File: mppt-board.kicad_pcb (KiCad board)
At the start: 6 copper layers, 46.5 x 49 mm, 29 parts, among them J1 Out, J2 programming, Q1 IPD25N06S4L30ATMA2, U1 MC33201DR2G, U2 LM3671, U3 STM32G030J6Mx

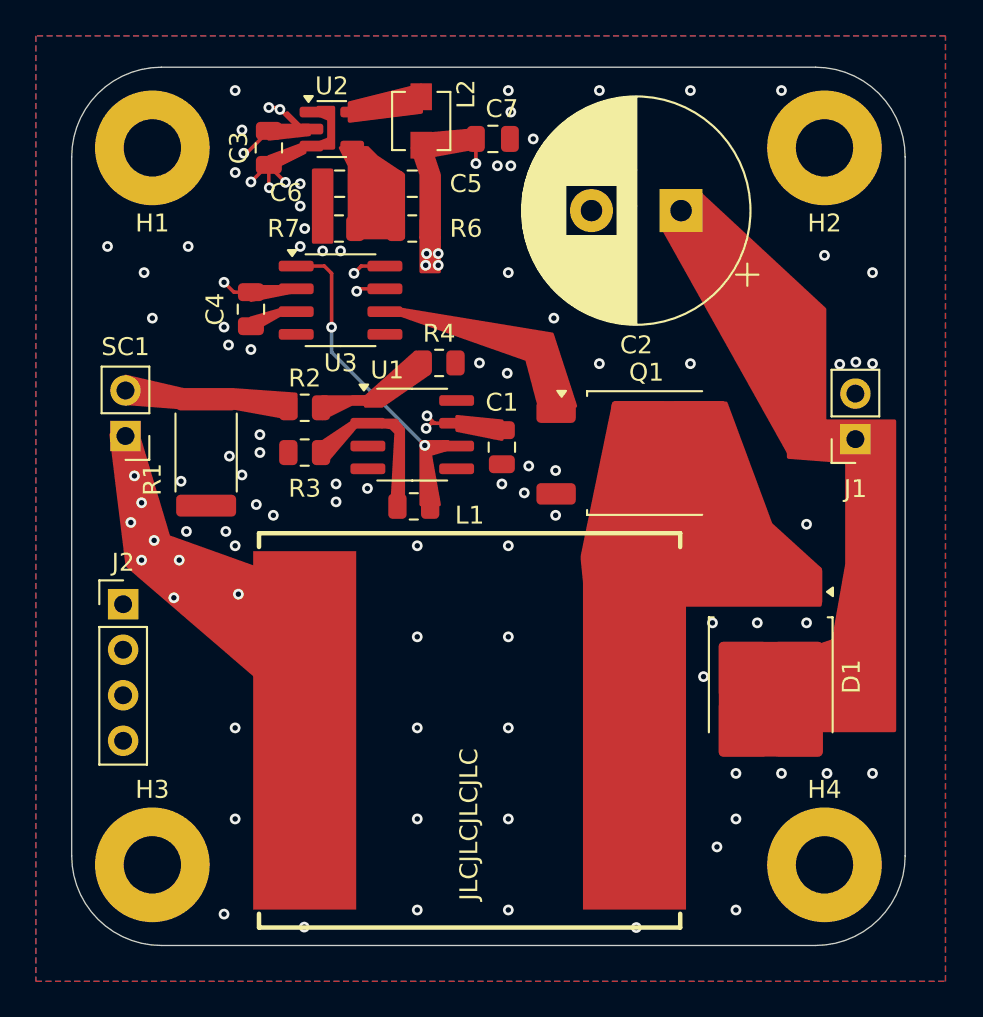
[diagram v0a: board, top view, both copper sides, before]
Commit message: init
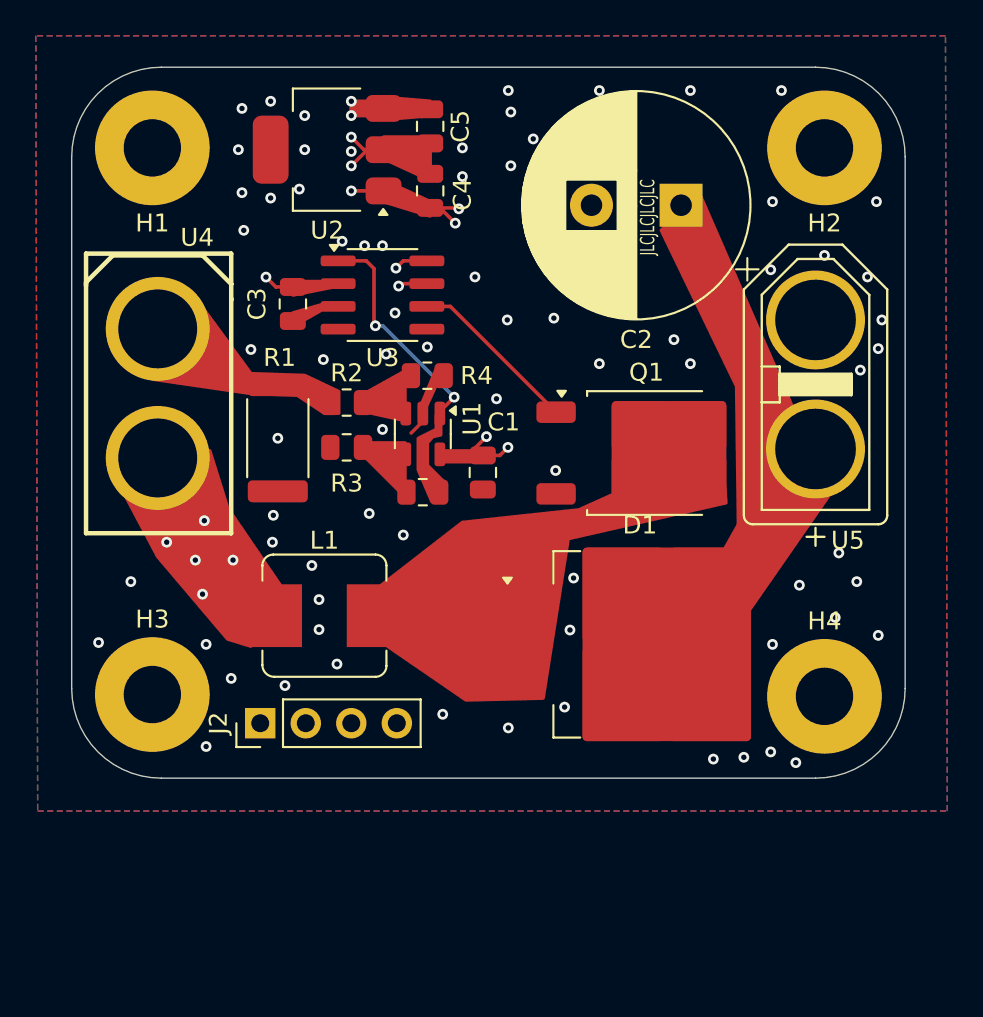
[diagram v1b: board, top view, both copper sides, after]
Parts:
- removed the C3 at (73.0, 54.0)
- removed C6: 33p, Capacitor_SMD:C_0805_2012Metric
- removed C7: 10u, Capacitor_SMD:C_0805_2012Metric
- removed J1: Out, Connector_PinSocket_2.54mm:PinSocket_1x02_P2.54mm_Vertical
- removed L2: 2.2u, Inductor_SMD:L_Vishay_IHLP-1212
- removed R6: 562k, Resistor_SMD:R_0805_2012Metric
- removed R7: 100k, Resistor_SMD:R_0805_2012Metric
- removed SC1: Solar_Cells, Connector_PinHeader_2.54mm:PinHeader_1x02_P2.54mm_Vertical
- added C4: 0.1u, Capacitor_SMD:C_0805_2012Metric, F.Cu at (82.0, 56.4)
- added U4: XT60, plib:CONN-TH_XT60, F.Cu at (66.8, 67.7)
- added U5: XT60-F, plib:CONN-TH_XT60PB-F, F.Cu at (103.5, 67.2)
- C5: value 6.8p -> 10u
- D1: footprint Package_TO_SOT_SMD:TO-252-2 -> Package_TO_SOT_SMD:TO-263-2
- L1: value FXL2213-680-M 100u -> MHCI06030-2R2M-R8; footprint plib:IND-SMD_L23.5-W22.0 -> Inductor_SMD:L_Bourns_SRP7028A_7.3x6.6mm
- R2, R3: value 282k -> 188k
- U1: value MC33201DR2G -> INA180A1; footprint Package_SO:SOIC-8_3.9x4.9mm_P1.27mm -> Package_TO_SOT_SMD:SOT-23-5
- U2: value LM3671 -> LM2937xMP; footprint Package_TO_SOT_SMD:TSOT-23-5 -> Package_TO_SOT_SMD:SOT-223-3_TabPin2
- moved L1 10.3 mm to (76.1, 80.1)
- moved J2 10.1 mm to (72.5, 86.1), turned to 90 degrees
- moved H3 9.50 mm to (66.5, 84.5)
- moved H4 9.40 mm to (104.0, 84.6)
- moved D1 7.52 mm to (93.7, 81.7), turned to 0 degrees
- moved R1 4.08 mm to (73.5, 70.2)
- moved C5 3.35 mm to (82.0, 52.8), turned to -90 degrees
- moved R2 2.36 mm to (77.3, 68.2)
- moved R3 2.36 mm to (77.3, 70.7)
- moved C3 2.36 mm to (74.3, 62.7)
- moved U3 2.36 mm to (79.3, 62.2)
- moved C1 1.76 mm to (84.9, 72.1)
- moved REF** 1.30 mm to (85.4, 67.3)
- moved U2 1.18 mm to (76.2, 54.1), turned to 180 degrees
- moved R4 0.97 mm to (81.8, 66.7)
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- renumbered C4 to C3
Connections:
- C5 pad 2: Net-(U2-FB) -> GND
- U1 pad 1: Net-(U1-+) -> /V_{drop}
- U1 pad 2: Net-(U1--) -> GND
- U1 pad 3: unconnected-(U1-Pad3) -> Net-(U1-+)
- U1 pad 4: GND -> Net-(U1--)
- U1 pad 5: unconnected-(U1-Pad5) -> VBUS
- U2 pad 3: VBUS -> VCC
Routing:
- net /pwm: track 0.00 -> 9.65 mm
- net VCC: track 3.10 -> 11.2 mm, vias 6 -> 3
- net /swdio: track 31.0 -> 27.1 mm
- net /V_{drop}: track 15.7 -> 12.7 mm
- net VBUS: track 6.44 -> 8.61 mm, vias 13 -> 10
- net GND: track 6.51 -> 5.62 mm, vias 91 -> 85
- removed copper zone on In3.Cu, net GND
- removed copper zone on In4.Cu, net GND
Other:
- board size 46.5 x 49 mm -> 46.5 x 39.7 mm
- copper layers 6 -> 4
